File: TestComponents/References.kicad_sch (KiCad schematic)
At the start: 15 parts, among them U13 X, U8 ADR510, U9 LM4040B

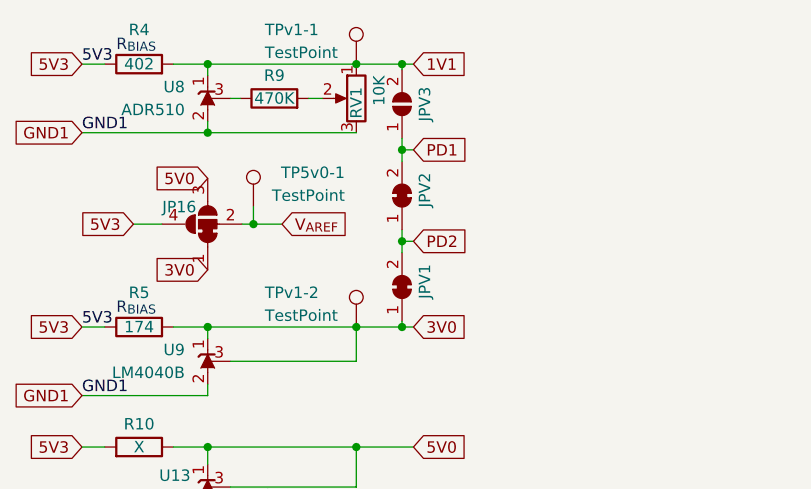
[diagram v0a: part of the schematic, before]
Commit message: SpectDrone Development
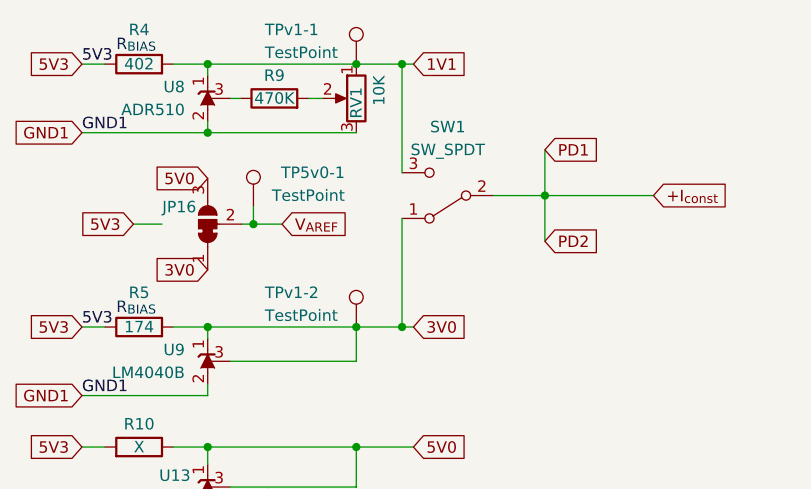
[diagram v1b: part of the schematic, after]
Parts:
- removed JPV1, JPV2: SolderJumper_2_Bridged, Jumper:SolderJumper-2_P1.3mm_Bridged_RoundedPad1.0x1.5mm, symbol Jumper:SolderJumper_2_Bridged
- removed JPV3: SolderJumper_2_Open, Jumper:SolderJumper-2_P1.3mm_Open_RoundedPad1.0x1.5mm, symbol Jumper:SolderJumper_2_Open
- added SW1: SW_SPDT, Button_Switch_SMD:SW_SPDT_CK-JS102011SAQN, symbol Switch:SW_SPDT
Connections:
- net 1V1: now also SW1.3 (C)
- net 3V0: now also SW1.1 (A)
- net 5V3: no longer JP16.4 (B)
- new net +I_{const}: SW1.2 (B)
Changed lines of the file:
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@@
   (junction (at 172.72 71.755) (diameter 0) (color 0 0 0 0)
   )
-  (junction (at 172.72 91.44) (diameter 0) (color 0 0 0 0)
-  )
   (junction (at 151.13 79.375) (diameter 0) (color 0 0 0 0)
   )
@@
   (junction (at 156.21 89.535) (diameter 0) (color 0 0 0 0)
   )
-  (junction (at 172.72 81.28) (diameter 0) (color 0 0 0 0)
+  (junction (at 188.595 86.36) (diameter 0) (color 0 0 0 0)
   )
   (junction (at 151.13 100.965) (diameter 0) (color 0 0 0 0)
@@
     (stroke (width 0) (type default) (color 0 0 0 0))
   )
-  (wire (pts (xy 172.72 100.33) (xy 172.72 100.965))
+  (wire (pts (xy 172.72 88.9) (xy 172.72 100.965))
     (stroke (width 0) (type default) (color 0 0 0 0))
   )
@@
     (stroke (width 0) (type default) (color 0 0 0 0))
   )
+  (wire (pts (xy 188.595 86.36) (xy 188.595 91.44))
+    (stroke (width 0) (type default) (color 0 0 0 0))
+  )
   (wire (pts (xy 137.16 121.92) (xy 151.13 121.92))
     (stroke (width 0) (type default) (color 0 0 0 0))
@@
     (stroke (width 0) (type default) (color 0 0 0 0))
   )
-  (wire (pts (xy 172.72 71.755) (xy 172.72 72.39))
+  (wire (pts (xy 172.72 71.755) (xy 172.72 83.82))
     (stroke (width 0) (type default) (color 0 0 0 0))
   )
@@
     (stroke (width 0) (type default) (color 0 0 0 0))
   )
-  (wire (pts (xy 172.72 81.28) (xy 173.99 81.28))
-    (stroke (width 0) (type default) (color 0 0 0 0))
-  )
   (wire (pts (xy 167.64 100.965) (xy 172.72 100.965))
     (stroke (width 0) (type default) (color 0 0 0 0))
   )
-  (wire (pts (xy 172.72 81.28) (xy 172.72 82.55))
-    (stroke (width 0) (type default) (color 0 0 0 0))
-  )
-  (wire (pts (xy 172.72 80.01) (xy 172.72 81.28))
-    (stroke (width 0) (type default) (color 0 0 0 0))
-  )
-  (wire (pts (xy 172.72 91.44) (xy 172.72 92.71))
-    (stroke (width 0) (type default) (color 0 0 0 0))
-  )
-  (wire (pts (xy 172.72 91.44) (xy 173.99 91.44))
-    (stroke (width 0) (type default) (color 0 0 0 0))
-  )
   (wire (pts (xy 147.32 100.965) (xy 151.13 100.965))
     (stroke (width 0) (type default) (color 0 0 0 0))
@@
     (stroke (width 0) (type default) (color 0 0 0 0))
   )
+  (wire (pts (xy 182.88 86.36) (xy 188.595 86.36))
+    (stroke (width 0) (type default) (color 0 0 0 0))
+  )
   (wire (pts (xy 156.21 87.63) (xy 156.21 89.535))
     (stroke (width 0) (type default) (color 0 0 0 0))
@@
     (stroke (width 0) (type default) (color 0 0 0 0))
   )
+  (wire (pts (xy 188.595 86.36) (xy 200.66 86.36))
+    (stroke (width 0) (type default) (color 0 0 0 0))
+  )
   (wire (pts (xy 137.16 114.3) (xy 139.7 114.3))
     (stroke (width 0) (type default) (color 0 0 0 0))
   )
-  (wire (pts (xy 172.72 90.17) (xy 172.72 91.44))
-    (stroke (width 0) (type default) (color 0 0 0 0))
-  )
   (wire (pts (xy 137.16 100.965) (xy 139.7 100.965))
     (stroke (width 0) (type default) (color 0 0 0 0))
@@
     (stroke (width 0) (type default) (color 0 0 0 0))
   )
+  (wire (pts (xy 188.595 81.28) (xy 188.595 86.36))
+    (stroke (width 0) (type default) (color 0 0 0 0))
+  )
   (wire (pts (xy 151.13 71.755) (xy 167.64 71.755))
     (stroke (width 0) (type default) (color 0 0 0 0))
@@
     )
   )
-  (global_label "PD2" (shape input) (at 173.99 91.44 0) (fields_autoplaced)
-    (effects (font (size 1.27 1.27)) (justify left))
-    (property "Intersheet References" "${INTERSHEET_REFS}" (id 0) (at 180.1526 91.3606 0)
+  (global_label "PD2" (shape input) (at 188.595 91.44 0) (fields_autoplaced)
+    (effects (font (size 1.27 1.27)) (justify left))
+    (property "Intersheet References" "${INTERSHEET_REFS}" (id 0) (at 194.7576 91.3606 0)
       (effects (font (size 1.27 1.27)) (justify left) hide)
     )
@@
     )
   )
+  (global_label "+I_{const}" (shape input) (at 200.66 86.36 0) (fields_autoplaced)
+    (effects (font (size 1.27 1.27)) (justify left))
+    (property "Intersheet References" "${INTERSHEET_REFS}" (id 0) (at 209.3626 86.4394 0)
+      (effects (font (size 1.27 1.27)) (justify left) hide)
+    )
+  )
   (global_label "GND_{RF}" (shape input) (at 137.16 121.92 180) (fields_autoplaced)
     (effects (font (size 1.27 1.27)) (justify right))
@@
     )
   )
-  (global_label "PD1" (shape input) (at 173.99 81.28 0) (fields_autoplaced)
-    (effects (font (size 1.27 1.27)) (justify left))
-    (property "Intersheet References" "${INTERSHEET_REFS}" (id 0) (at 180.1526 81.2006 0)
+  (global_label "PD1" (shape input) (at 188.595 81.28 0) (fields_autoplaced)
+    (effects (font (size 1.27 1.27)) (justify left))
+    (property "Intersheet References" "${INTERSHEET_REFS}" (id 0) (at 194.7576 81.2006 0)
       (effects (font (size 1.27 1.27)) (justify left) hide)
     )
@@
     (pin "2")
   )
-  (symbol (lib_id "Jumper:SolderJumper_2_Bridged") (at 172.72 86.36 90) (unit 1)
-    (in_bom yes) (on_board yes)
-    (property "Reference" "JPV2" (id 0) (at 175.26 83.82 0)
-      (effects (font (size 1.27 1.27)) (justify right))
-    )
-    (property "Value" "SolderJumper_2_Bridged" (id 1) (at 175.26 87.6299 90)
-      (effects (font (size 1.27 1.27)) (justify right) hide)
-    )
-    (property "Footprint" "Jumper:SolderJumper-2_P1.3mm_Bridged_RoundedPad1.0x1.5mm" (id 2) (at 172.72 86.36 0)
-      (effects (font (size 1.27 1.27)) hide)
-    )
-    (property "Datasheet" "~" (id 3) (at 172.72 86.36 0)
-      (effects (font (size 1.27 1.27)) hide)
-    )
-    (pin "1")
-    (pin "2")
+  (symbol (lib_id "Switch:SW_SPDT") (at 177.8 86.36 180) (unit 1)
+    (in_bom yes) (on_board yes) (fields_autoplaced)
+    (property "Reference" "SW1" (id 0) (at 177.8 78.74 0))
+    (property "Value" "SW_SPDT" (id 1) (at 177.8 81.28 0))
+    (property "Footprint" "Button_Switch_SMD:SW_SPDT_CK-JS102011SAQN" (id 2) (at 177.8 86.36 0)
+      (effects (font (size 1.27 1.27)) hide)
+    )
+    (property "Datasheet" "~" (id 3) (at 177.8 86.36 0)
+      (effects (font (size 1.27 1.27)) hide)
+    )
+    (pin "1")
+    (pin "2")
+    (pin "3")
   )
   (symbol (lib_id "Device:R") (at 143.51 100.965 90) (unit 1)
@@
     (pin "2")
     (pin "3")
-    (pin "4")
-  )
-  (symbol (lib_id "Jumper:SolderJumper_2_Bridged") (at 172.72 96.52 90) (unit 1)
-    (in_bom yes) (on_board yes)
-    (property "Reference" "JPV1" (id 0) (at 175.26 93.98 0)
-      (effects (font (size 1.27 1.27)) (justify right))
-    )
-    (property "Value" "SolderJumper_2_Bridged" (id 1) (at 175.26 97.7899 90)
-      (effects (font (size 1.27 1.27)) (justify right) hide)
-    )
-    (property "Footprint" "Jumper:SolderJumper-2_P1.3mm_Bridged_RoundedPad1.0x1.5mm" (id 2) (at 172.72 96.52 0)
-      (effects (font (size 1.27 1.27)) hide)
-    )
-    (property "Datasheet" "~" (id 3) (at 172.72 96.52 0)
-      (effects (font (size 1.27 1.27)) hide)
-    )
-    (pin "1")
-    (pin "2")
   )
   (symbol (lib_id "Gardenuino_Custom:ADR510") (at 151.13 118.745 270) (mirror x) (unit 1)
@@
     (pin "1")
   )
-  (symbol (lib_id "Jumper:SolderJumper_2_Open") (at 172.72 76.2 90) (unit 1)
-    (in_bom yes) (on_board yes)
-    (property "Reference" "JPV3" (id 0) (at 175.26 76.2 0))
-    (property "Value" "SolderJumper_2_Open" (id 1) (at 175.26 69.85 0)
-      (effects (font (size 1.27 1.27)) hide)
-    )
-    (property "Footprint" "Jumper:SolderJumper-2_P1.3mm_Open_RoundedPad1.0x1.5mm" (id 2) (at 172.72 76.2 0)
-      (effects (font (size 1.27 1.27)) hide)
-    )
-    (property "Datasheet" "~" (id 3) (at 172.72 76.2 0)
-      (effects (font (size 1.27 1.27)) hide)
-    )
-    (pin "1")
-    (pin "2")
-  )
 )

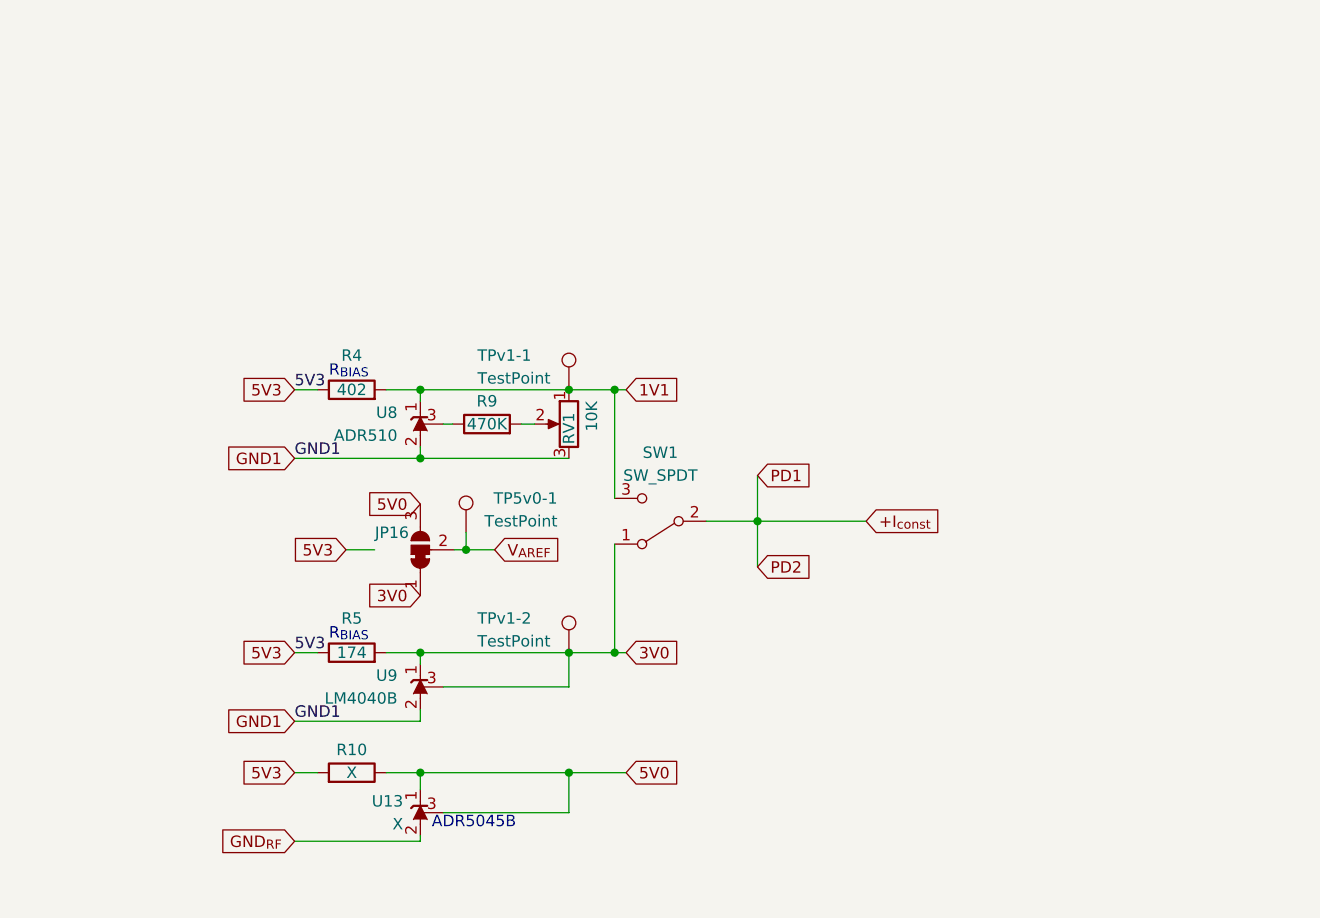
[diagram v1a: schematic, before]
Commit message: SpectDrone Development
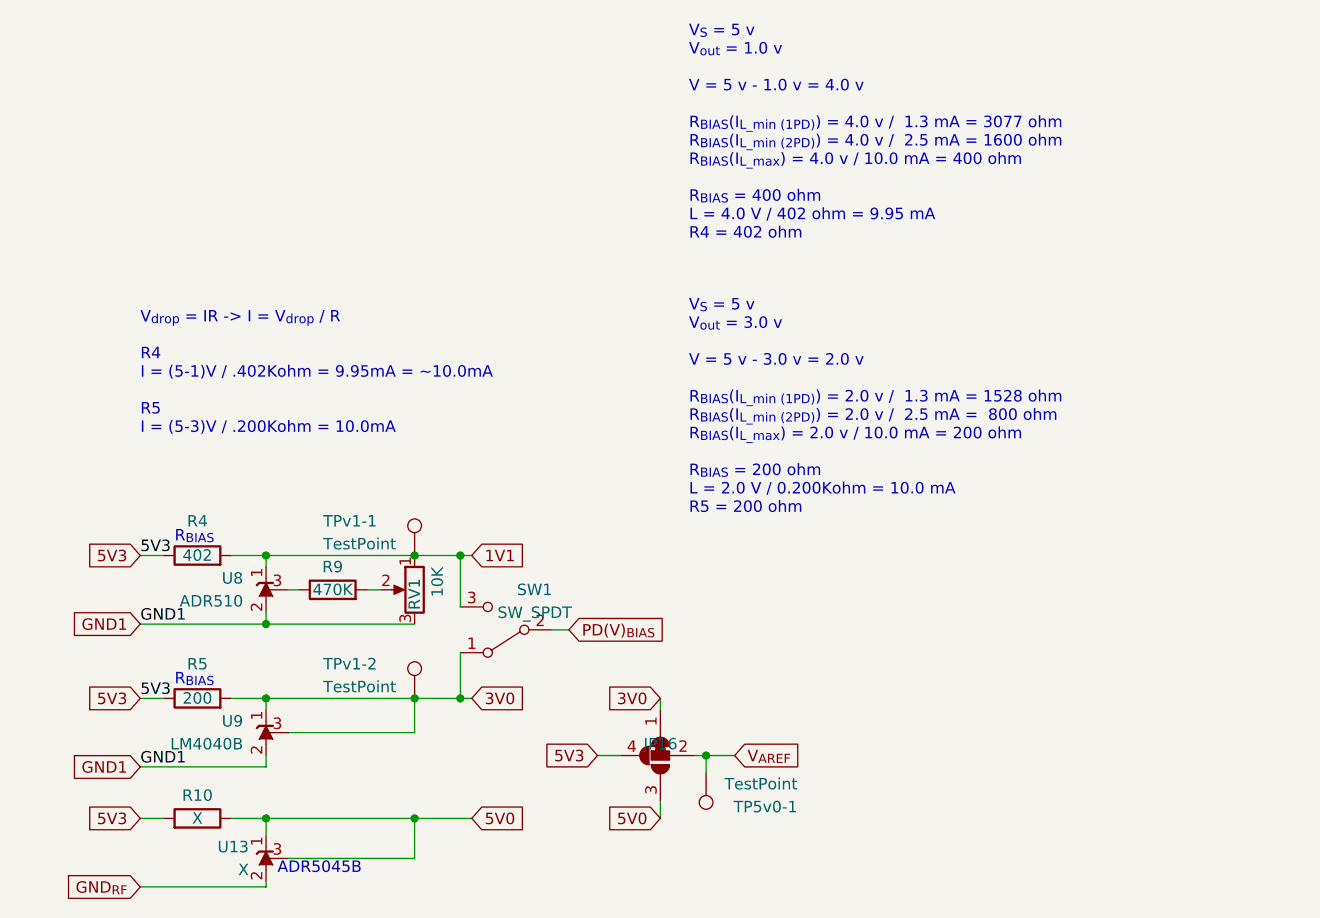
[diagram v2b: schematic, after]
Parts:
- R5: value 174 -> 200
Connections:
- net 5V3: now also JP16.4
- net +I_{const} renamed PD(V)_{BIAS}
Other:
- note added: "V_{S} = 5 v V_{out} = 1.0 v V = 5 v - 1.0 v = 4.0 v R_{BIAS}(I_{L_min (1PD)}) = 4.0 v / 1.3 mA = 3077 ohm R_{BIAS}(I_{L_min (2PD)}) = 4.0 v / 2.5 mA = 1600 ohm R_{BIAS}(I_{L_max}) = 4.0 v / 10.0 mA = 400 ohm R_{BIAS} = 400 ohm L = 4.0 V / 402 ohm = 9.95 mA R4 = 402 ohm"
- note added: "V_{S} = 5 v V_{out} = 3.0 v V = 5 v - 3.0 v = 2.0 v R_{BIAS}(I_{L_min (1PD)}) = 2.0 v / 1.3 mA = 1528 ohm R_{BIAS}(I_{L_min (2PD)}) = 2.0 v / 2.5 mA = 800 ohm R_{BIAS}(I_{L_max}) = 2.0 v / 10.0 mA = 200 ohm R_{BIAS} = 200 ohm L = 2.0 V / 0.200Kohm = 10.0 mA R5 = 200 ohm"
- note added: "V_{drop} = IR -> I = V_{drop} / R R4 I = (5-1)V / .402Kohm = 9.95mA = ~10.0mA R5 I = (5-3)V / .200Kohm = 10.0mA"
- moved on the sheet: R10, R4, R5, R9, RV1, SW1, TP5v0-1, TPv1-1, TPv1-2, U13, U8, U9

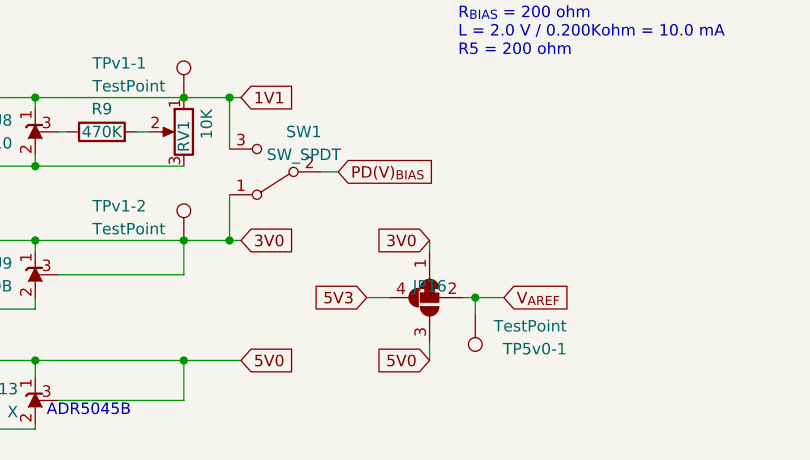
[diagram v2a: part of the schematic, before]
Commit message: SpectDrone Development
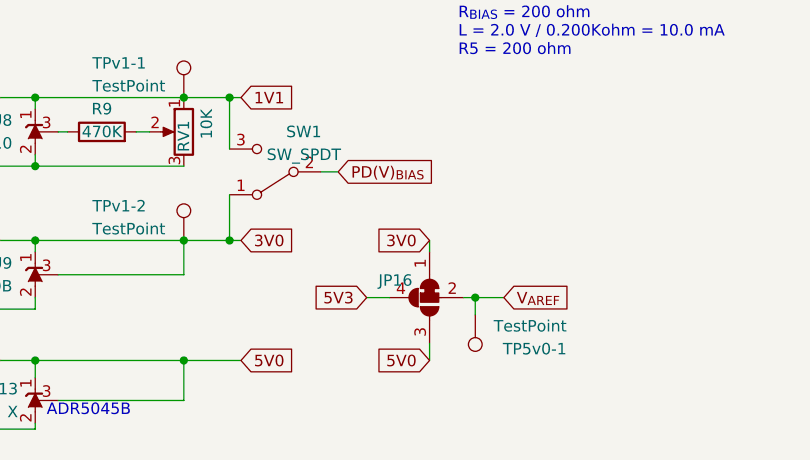
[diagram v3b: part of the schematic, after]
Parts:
- RV1: footprint Potentiometer_THT:Potentiometer_Bourns_3296W_Vertical -> Potentiometer_THT:Potentiometer_Bourns_3296P_Horizontal
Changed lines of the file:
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@@
   (symbol (lib_id "Jumper:SolderJumper_3_Bridged12") (at 177.8 112.395 90) (mirror x) (unit 1)
     (in_bom yes) (on_board yes)
-    (property "Reference" "JP16" (id 0) (at 179.705 111.125 90)
+    (property "Reference" "JP16" (id 0) (at 175.895 110.49 90)
       (effects (font (size 1.27 1.27)) (justify left))
     )
@@
       (effects (font (size 1.27 1.27)) (justify right))
     )
-    (property "Footprint" "Potentiometer_THT:Potentiometer_Bourns_3296W_Vertical" (id 2) (at 150.495 93.98 0)
+    (property "Footprint" "Potentiometer_THT:Potentiometer_Bourns_3296P_Horizontal" (id 2) (at 150.495 93.98 0)
       (effects (font (size 1.27 1.27)) hide)
     )

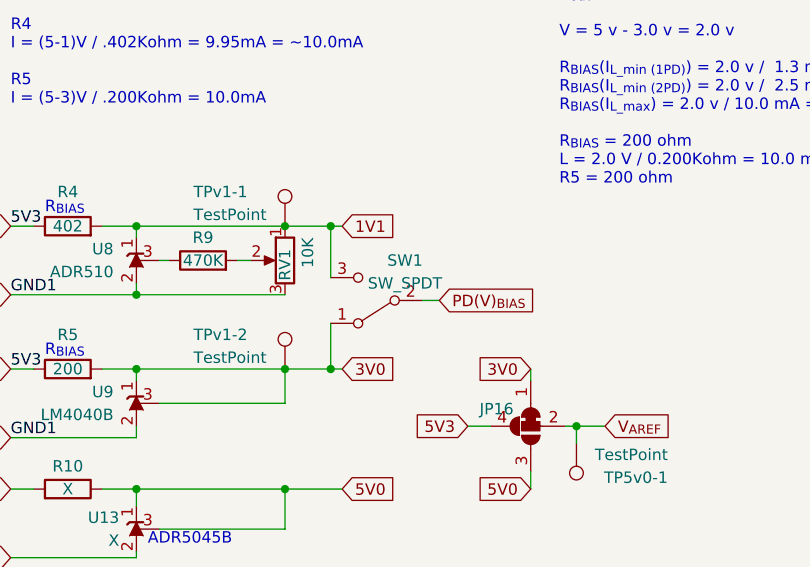
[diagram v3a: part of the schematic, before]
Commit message: SpectDrone Development
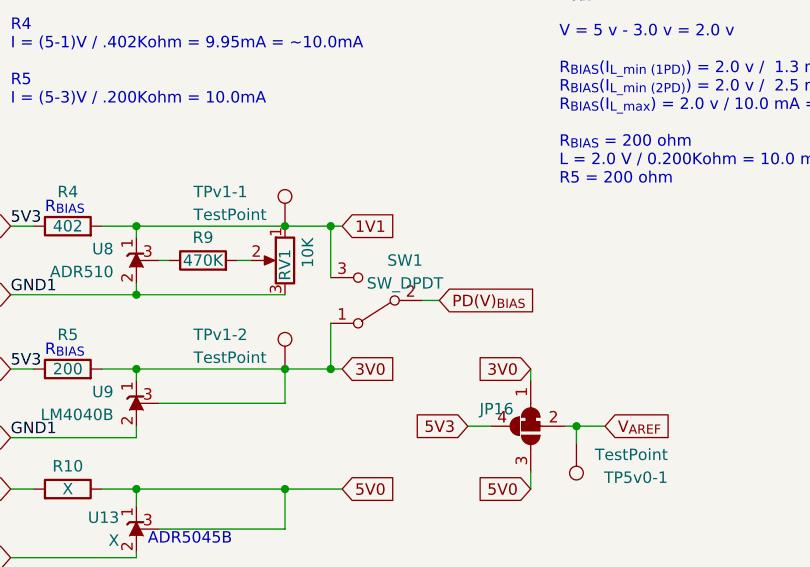
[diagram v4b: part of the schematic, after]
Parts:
- SW1: value SW_SPDT -> SW_DPDT; footprint Button_Switch_SMD:SW_SPDT_CK-JS102011SAQN -> Gardenuino Custom:SW_DPDT_CK_JS202011JAQN
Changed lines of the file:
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@@
     (in_bom yes) (on_board yes)
     (property "Reference" "SW1" (id 0) (at 163.83 93.98 0))
-    (property "Value" "SW_SPDT" (id 1) (at 163.83 96.52 0))
-    (property "Footprint" "Button_Switch_SMD:SW_SPDT_CK-JS102011SAQN" (id 2) (at 160.655 98.425 0)
+    (property "Value" "SW_DPDT" (id 1) (at 163.83 96.52 0))
+    (property "Footprint" "Gardenuino Custom:SW_DPDT_CK_JS202011JAQN" (id 2) (at 160.655 98.425 0)
       (effects (font (size 1.27 1.27)) hide)
     )
